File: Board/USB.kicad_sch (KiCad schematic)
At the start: 29 parts, among them IC8 MAX3421E, Q2 32kHz, Q3 12MHz

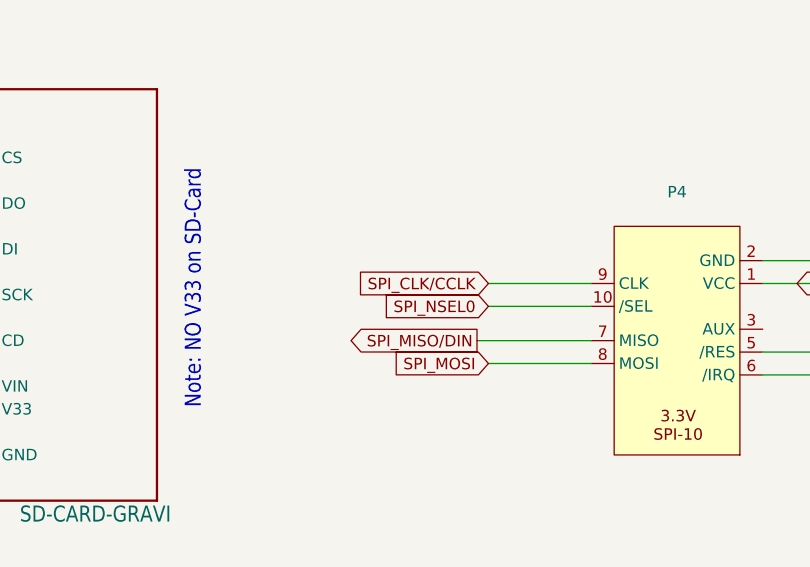
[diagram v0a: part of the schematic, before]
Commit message: more work on 1.3
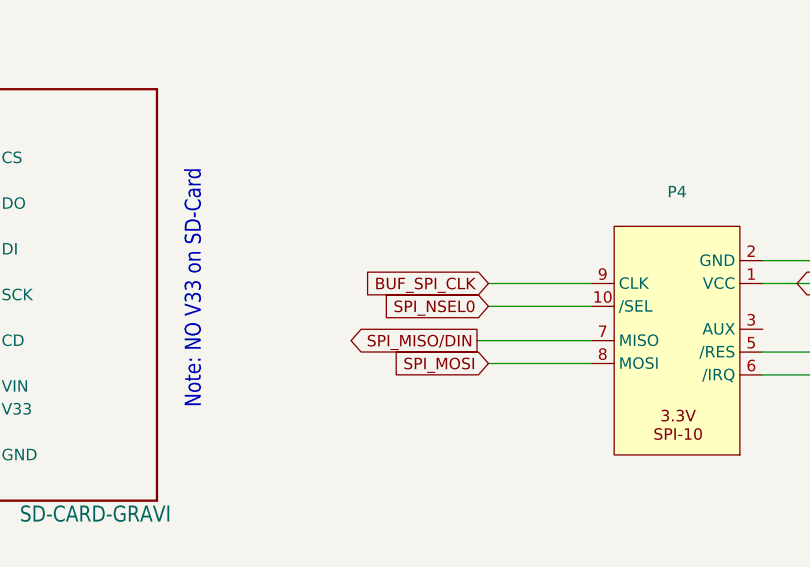
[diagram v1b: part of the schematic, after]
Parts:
- IC8: footprint cbm_ultipet_v1:TQFP32-5MM -> Package_QFP:LQFP-32_5x5mm_P0.5mm
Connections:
- net SPI_CLK/CCLK: no longer P4.9 (CLK)
- new net BUF_SPI_CLK: P4.9 (CLK)
